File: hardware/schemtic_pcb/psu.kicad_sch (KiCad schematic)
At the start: 25 parts, among them J5 Conn_01x06, Q1 IRF520N, Q2 2N7002, U1 ACS712xLCTR-05B, U2 LM2576HVS-ADJ

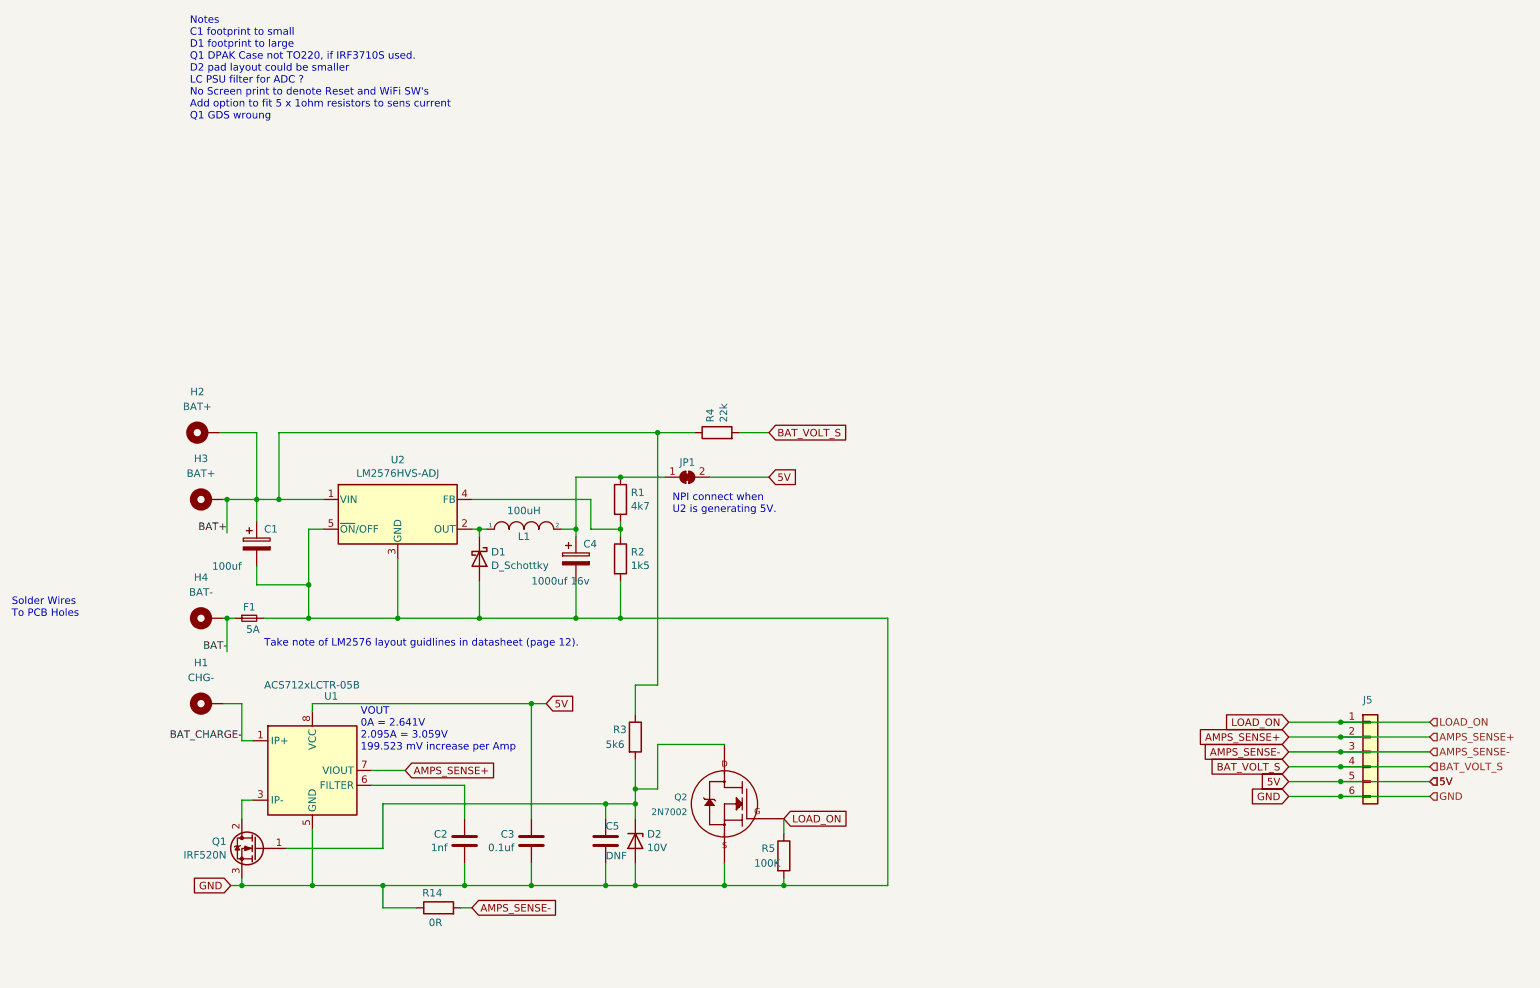
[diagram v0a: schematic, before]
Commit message: Bump schematic and PCB to version 3.0
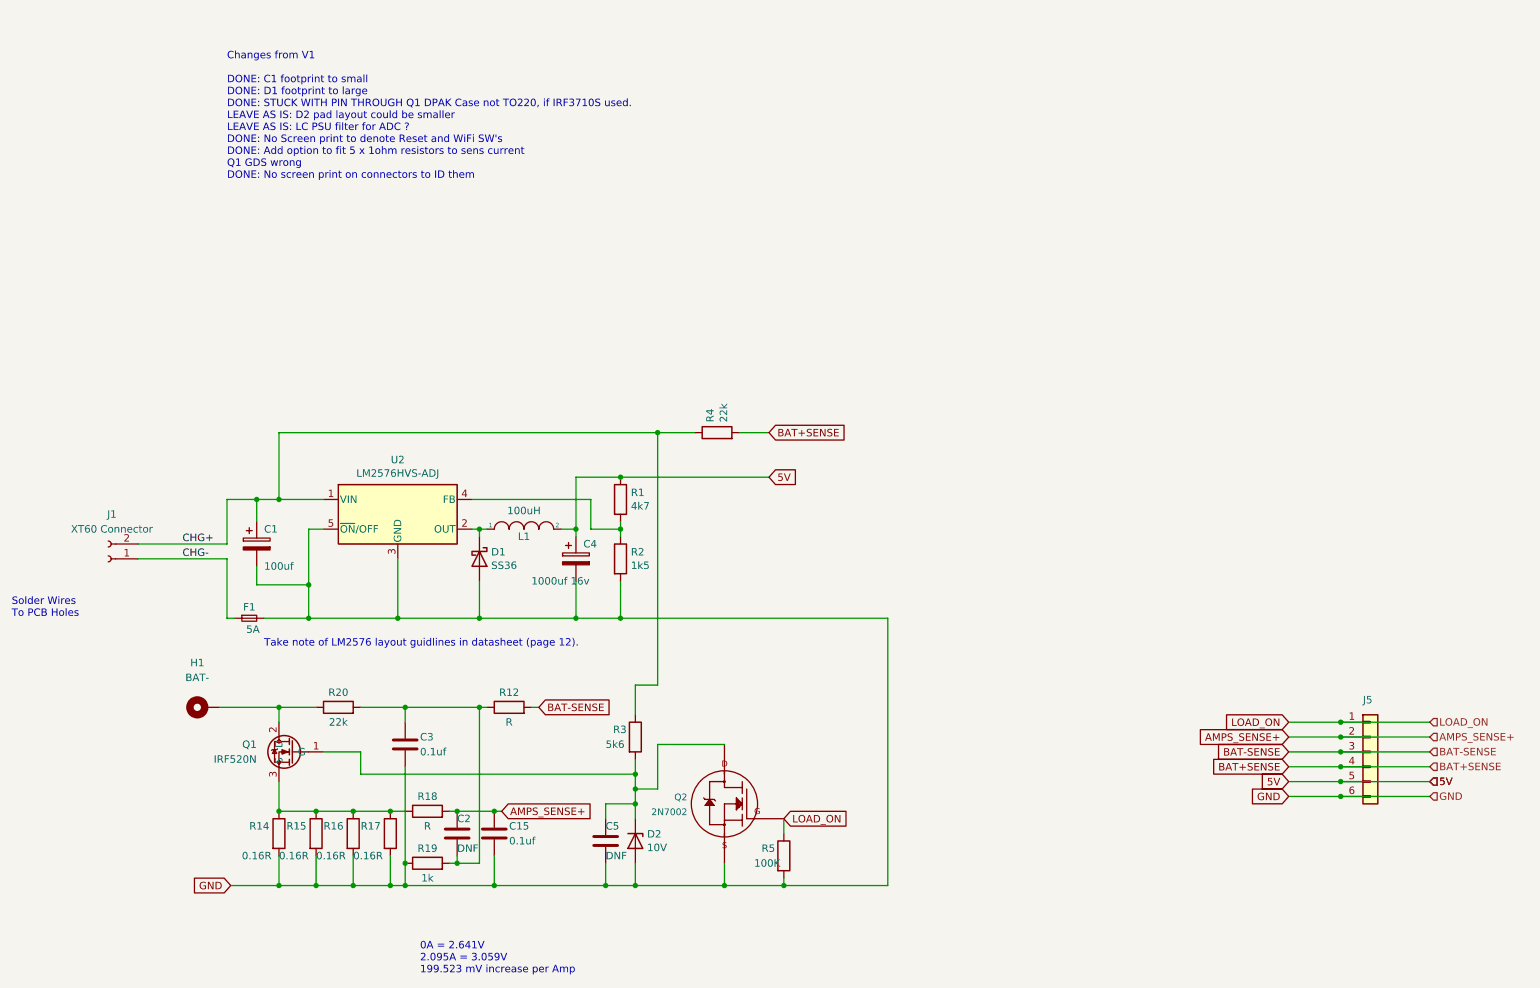
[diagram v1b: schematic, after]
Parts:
- removed H2, H3: BAT+, MountingHole:MountingHole_3.2mm_M3_Pad, symbol Mechanical:MountingHole_Pad
- removed H4: BAT-, MountingHole:MountingHole_3.2mm_M3_Pad, symbol Mechanical:MountingHole_Pad
- removed JP1: SolderJumper_2_Bridged, Jumper:SolderJumper-2_P1.3mm_Bridged_RoundedPad1.0x1.5mm, symbol Jumper:SolderJumper_2_Bridged
- removed Q1: IRF520N, Package_TO_SOT_THT:TO-220-3_Vertical, symbol Device:Q_NMOS_GDS
- removed U1: ACS712xLCTR-05B, Package_SO:SOIC-8_3.9x4.9mm_P1.27mm, symbol Sensor_Current:ACS712xLCTR-05B
- added C15: 0.1uf, Capacitor_SMD:C_0603_1608Metric_Pad1.08x0.95mm_HandSolder, symbol Device:C
- added J1: XT60 Connector, Connector_AMASS:AMASS_XT60-F_1x02_P7.20mm_Vertical, symbol Connector:Conn_01x02_Female
- added Q1: IRF520N, Package_TO_SOT_THT:TO-220-3_Vertical, symbol Transistor_FET:IRF540N
- added R12, R18: R, Resistor_SMD:R_0603_1608Metric_Pad0.98x0.95mm_HandSolder, symbol Device:R
- added R15, R16, R17: 0.16R, Resistor_SMD:R_1206_3216Metric_Pad1.30x1.75mm_HandSolder, symbol Device:R
- added R19: 1k, Resistor_SMD:R_0603_1608Metric_Pad0.98x0.95mm_HandSolder, symbol Device:R
- added R20: 22k, Resistor_SMD:R_0603_1608Metric_Pad0.98x0.95mm_HandSolder, symbol Device:R
- C1: footprint Capacitor_THT:CP_Radial_D5.0mm_P2.00mm -> Capacitor_THT:CP_Radial_D10.0mm_P5.00mm
- C2: value 1nf -> DNF
- D1: value D_Schottky -> SS36; footprint PJA_Semiconductors:SS34_DIODE_HANDSOLDER -> Diode_SMD:D_MELF
- H1: value CHG- -> BAT-
- Q2: footprint Package_TO_SOT_SMD:SOT-23 -> Package_TO_SOT_SMD:TSOT-23
- R14: value 0R -> 0.16R; footprint Resistor_SMD:R_0603_1608Metric_Pad0.98x0.95mm_HandSolder -> Resistor_SMD:R_1206_3216Metric_Pad1.30x1.75mm_HandSolder
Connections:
- net 5V: now also C4.1, L1.2, R1.1; no longer C3.1
- net AMPS_SENSE+: now also C2.1, C15.1, R18.2
- net GND: now also R14.2, C15.2, R15.2, R16.2, R17.2, R19.1; no longer C2.2, R14.1
- net at C5.1, D2.1 (K), Q2.3 (D)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: now also Q1.1 (G)
- net AMPS_SENSE- renamed BAT-SENSE
- net BAT-SENSE: now also R12.2; no longer R14.2
- net BAT+ renamed CHG+
- net CHG+: now also J1.2 (Pin_2)
- net BAT- renamed CHG-
- net CHG-: now also J1.1 (Pin_1)
- net BAT_CHARGE-: no longer names the net of H1.1
- net BAT_CHARGE-: now also Q1.2 (D), R20.1
- net BAT_VOLT_S renamed BAT+SENSE
- new net: Q1.3 (S), R14.1, R15.1, R16.1, R17.1, R18.1
- new net: C2.2, C3.1, R12.1, R19.2, R20.2
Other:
- note added: "0A = 2.641V 2.095A = 3.059V 199.523 mV increase per Amp"
- note added: "Changes from V1 DONE: C1 footprint to small DONE: D1 footprint to large DONE: STUCK WITH PIN THROUGH Q1 DPAK Case not TO220, if IRF3710S used. LEAVE AS IS: D2 pad layout could be smaller LEAVE AS IS: LC PSU filter for ADC ? DONE: No Screen print to denote Reset and WiFi SW's DONE: Add option to fit 5 x 1ohm resistors to sens current Q1 GDS wrong DONE: No screen print on connectors to ID them"
- note removed: "NPI connect when U2 is generating 5V."
- note removed: "Notes C1 footprint to small D1 footprint to large Q1 DPAK Case not TO220, if IRF3710S used. D2 pad layout could be smaller LC PSU filter for ADC ? No Screen print to denote Reset and WiFi SW's Add option to fit 5 x 1ohm resistors to sens current Q1 GDS wroung"
- note removed: "VOUT 0A = 2.641V 2.095A = 3.059V 199.523 mV increase per Amp"
- moved on the sheet: H1
